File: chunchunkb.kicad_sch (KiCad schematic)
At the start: 124 parts, among them J1 BATT, J2 OLED, SW1 SW_Push, SW10 SW_Push, SW11 SW_Push, SW12 SW_Push, SW13 SW_Push, SW14 SW_Push, SW15 SW_Push, SW16 SW_Push, SW17 SW_Push, SW18 SW_Push, SW19 SW_Push, SW2 SW_Push, SW20 SW_Push, SW21 SW_Push, SW22 SW_Push, SW23 SW_Push, SW24 SW_Push, SW25 SW_Push, SW26 SW_Push, SW27 SW_Push, SW28 SW_Push, SW29 SW_Push, SW3 SW_Push, SW30 SW_Push, SW31 EC11, SW32 SW_Push, SW33 SW_Push, SW34 SW_Push, SW35 SW_Push, SW36 SW_Push, SW4 SW_Push, SW5 SW_Push, SW6 SW_Push, SW7 SW_Push, SW8 SW_Push, SW9 SW_Push

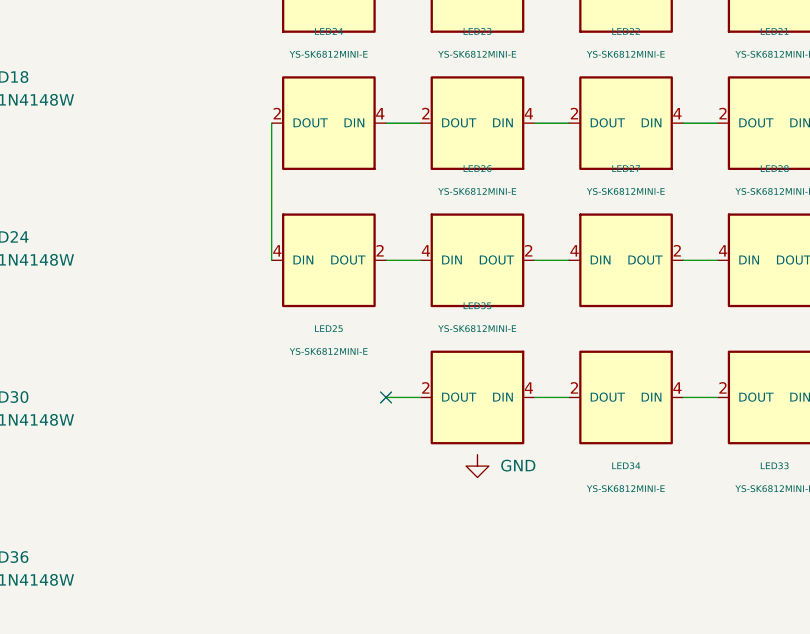
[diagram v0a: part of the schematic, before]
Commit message: Merge pull request #2 from qwerty22121998/feat/rev2
feat: rev 2 board
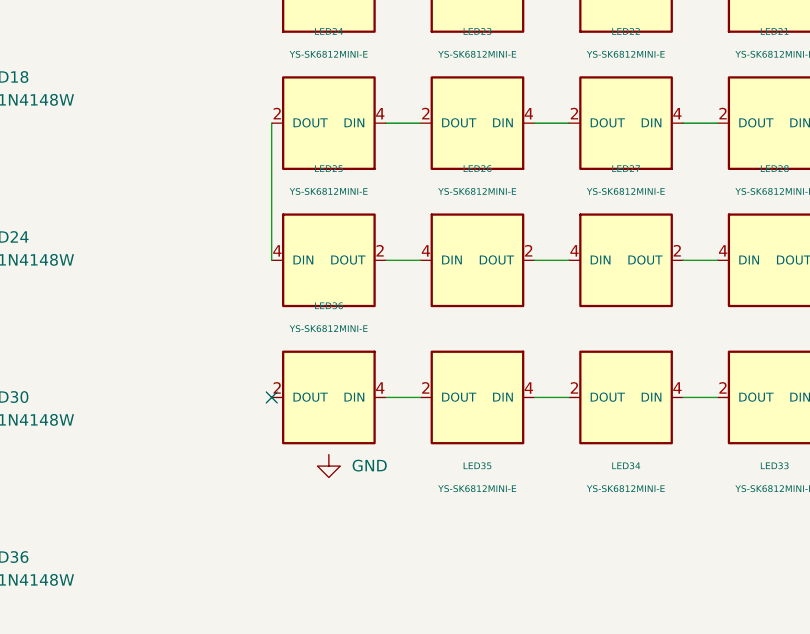
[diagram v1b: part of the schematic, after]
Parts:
- added LED36: YS-SK6812MINI-E, chunchunkb:YS-SK6812MINI-E, symbol kbd:YS-SK6812MINI-E
- SW31: footprint chunchunkb:EC11_Switch -> chunchunkb:EC11_MX_Hybrid
- U1: footprint chunchunkb:ProMicro DUAL -> chunchunkb:ProMicro_DUAL
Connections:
- net GND: now also LED36.3 (GND)
- net VCC: now also LED36.1 (VDD)
- net at LED35.2 (DOUT): now also LED36.4 (DIN)
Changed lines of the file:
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@@
 	)
 	(no_connect
-		(at 281.94 118.11)
+		(at 269.24 118.11)
 	)
 	(no_connect
@@
 	)
 	(symbol
+		(lib_name "YS-SK6812MINI-E_35")
+		(lib_id "kbd:YS-SK6812MINI-E")
+		(at 275.59 118.11 0)
+		(mirror y)
+		(unit 1)
+		(body_style 1)
+		(exclude_from_sim no)
+		(in_bom yes)
+		(on_board yes)
+		(in_pos_files yes)
+		(dnp no)
+		(fields_autoplaced yes)
+		(property "Reference" "LED36"
+			(at 275.59 107.95 0)
+			(show_name no)
+			(do_not_autoplace no)
+			(effects
+				(font
+					(size 0.7366 0.7366)
+				)
+			)
+		)
+		(property "Value" "YS-SK6812MINI-E"
+			(at 275.59 110.49 0)
+			(show_name no)
+			(do_not_autoplace no)
+			(effects
+				(font
+					(size 0.7366 0.7366)
+				)
+			)
+		)
+		(property "Footprint" "chunchunkb:YS-SK6812MINI-E"
+			(at 273.05 124.46 0)
+			(hide yes)
+			(show_name no)
+			(do_not_autoplace no)
+			(effects
+				(font
+					(size 1.27 1.27)
+				)
+			)
+		)
+		(property "Datasheet" ""
+			(at 273.05 124.46 0)
+			(hide yes)
+			(show_name no)
+			(do_not_autoplace no)
+			(effects
+				(font
+					(size 1.27 1.27)
+				)
+			)
+		)
+		(property "Description" ""
+			(at 275.59 118.11 0)
+			(hide yes)
+			(show_name no)
+			(do_not_autoplace no)
+			(effects
+				(font
+					(size 1.27 1.27)
+				)
+			)
+		)
+		(pin "1"
+		)
+		(pin "4"
+		)
+		(pin "3"
+		)
+		(pin "2"
+		)
+		(instances
+			(project "chunchunkb"
+				(path "/c64465b6-eb49-4a63-b501-311556755a54"
+					(reference "LED36")
+					(unit 1)
+				)
+			)
+		)
+	)
+	(symbol
 		(lib_id "Diode:1N4148W")
 		(at 208.28 83.82 270)
@@
 			)
 		)
-		(property "Footprint" "chunchunkb:ProMicro DUAL"
+		(property "Footprint" "chunchunkb:ProMicro_DUAL"
 			(at 102.87 115.57 90)
 			(hide yes)
@@
 			)
 		)
-		(property "Footprint" "chunchunkb:EC11_Switch"
+		(property "Footprint" "chunchunkb:EC11_MX_Hybrid"
 			(at 77.47 131.826 0)
 			(hide yes)
@@
 	(symbol
 		(lib_id "power:GND")
-		(at 292.1 124.46 0)
+		(at 275.59 124.46 0)
 		(mirror y)
 		(unit 1)
@@
 		(fields_autoplaced yes)
 		(property "Reference" "#PWR012"
-			(at 292.1 130.81 0)
+			(at 275.59 130.81 0)
 			(hide yes)
 			(show_name no)
@@
 		)
 		(property "Value" "GND"
-			(at 294.64 125.73 0)
+			(at 278.13 125.73 0)
 			(show_name no)
 			(do_not_autoplace no)
@@
 		)
 		(property "Footprint" ""
-			(at 292.1 124.46 0)
+			(at 275.59 124.46 0)
 			(hide yes)
 			(show_name no)
@@
 		)
 		(property "Datasheet" ""
-			(at 292.1 124.46 0)
+			(at 275.59 124.46 0)
 			(hide yes)
 			(show_name no)
@@
 		)
 		(property "Description" "Power symbol creates a global label with name \"GND\" , ground"
-			(at 292.1 124.46 0)
+			(at 275.59 124.46 0)
 			(hide yes)
 			(show_name no)
@@
 		(fields_autoplaced yes)
 		(property "Reference" "LED35"
-			(at 292.1 107.95 0)
+			(at 292.1 125.73 0)
 			(show_name no)
 			(do_not_autoplace no)
@@
 		)
 		(property "Value" "YS-SK6812MINI-E"
-			(at 292.1 110.49 0)
+			(at 292.1 128.27 0)
 			(show_name no)
 			(do_not_autoplace no)
@@
 		(fields_autoplaced yes)
 		(property "Reference" "LED25"
-			(at 275.59 110.49 0)
+			(at 275.59 92.71 0)
 			(show_name no)
 			(do_not_autoplace no)
@@
 		)
 		(property "Value" "YS-SK6812MINI-E"
-			(at 275.59 113.03 0)
+			(at 275.59 95.25 0)
 			(show_name no)
 			(do_not_autoplace no)
